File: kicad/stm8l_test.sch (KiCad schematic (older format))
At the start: 26 parts, among them J1 Conn_01x04, J2 Conn_01x02, Q1 2N7002, SW1 SW_Push, SW2 prog_sw, SW3 Rotary_Encoder_Switch, U2 STM8L101F3P, U3 BD70522GUL-E2

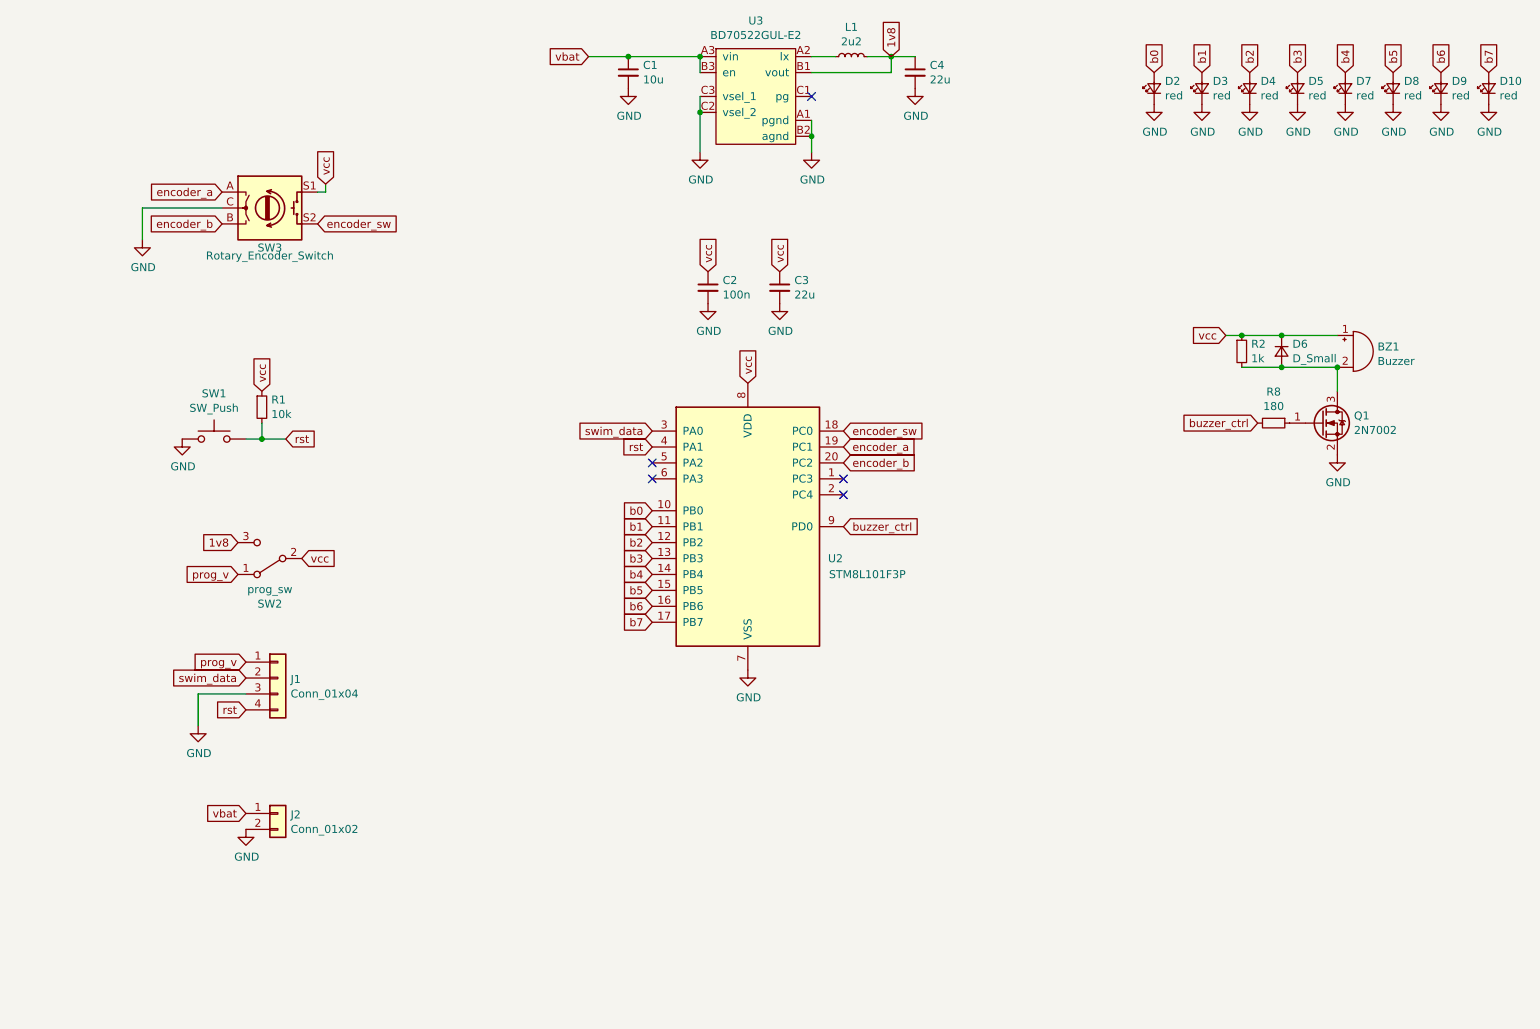
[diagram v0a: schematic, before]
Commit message: thinking about the solution, picking leds et al
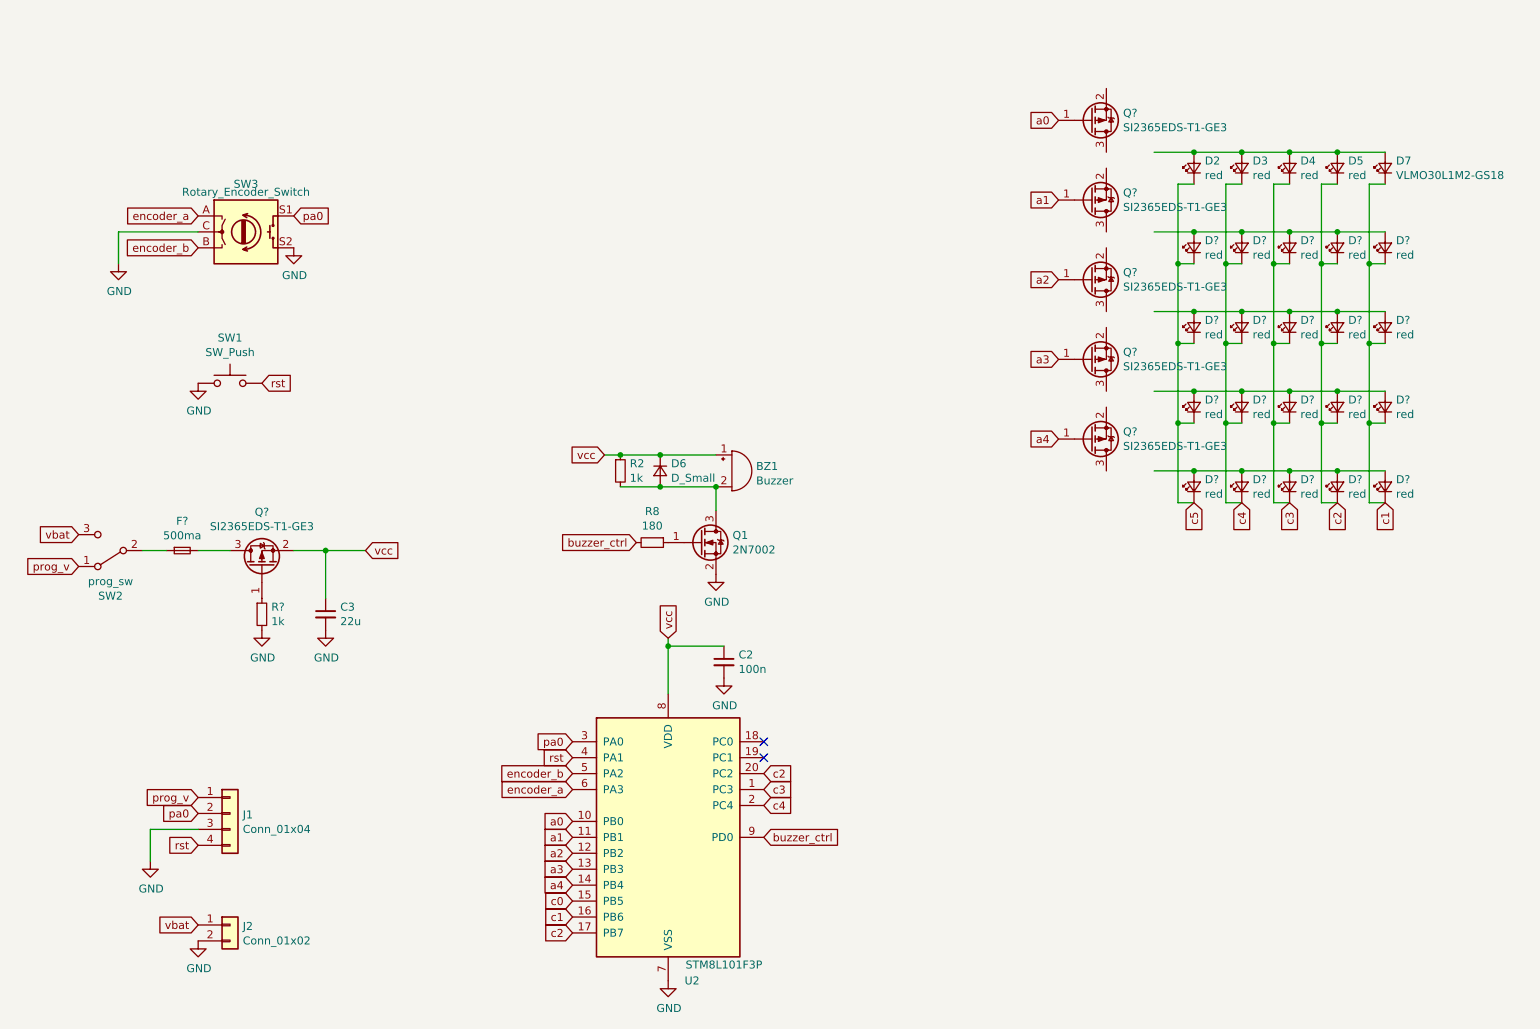
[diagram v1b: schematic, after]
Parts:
- removed C1: 10u, Capacitor_SMD:C_0805_2012Metric_Pad1.15x1.40mm_HandSolder, symbol Device:C_Small
- removed C4: 22u, Capacitor_SMD:C_0805_2012Metric_Pad1.15x1.40mm_HandSolder, symbol Device:C_Small
- removed D10, D8, D9: red, LED_SMD:LED_1206_3216Metric_Pad1.42x1.75mm_HandSolder, symbol Device:LED_Small
- removed L1: 2u2, Inductor_SMD:L_Wuerth_WE-PD-Typ-7345, symbol Device:L_Small
- removed R1: 10k, Resistor_SMD:R_0603_1608Metric_Pad1.05x0.95mm_HandSolder, symbol Device:R_Small
- removed U3: BD70522GUL-E2, good_things:BGA-9_3x3_1.76x1.56mm, symbol good_things:BD70522GUL-E2
- added D? (x20): red, LED_SMD:LED_1206_3216Metric_Pad1.42x1.75mm_HandSolder, symbol Device:LED_Small
- added F?: 500ma, symbol Device:Fuse_Small
- added Q? (x6): SI2365EDS-T1-GE3, symbol Device:Q_PMOS_GSD
- added R?: 1k, symbol Device:R_Small
- D7: value red -> VLMO30L1M2-GS18
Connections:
- net labels added: a0, a1, a2, a3, a4, c0, c1, c2, c3, c4, c5, pa0
- net labels removed: 1v8, b0, b1, b2, b3, b4, b5, b6, b7, encoder_sw, swim_data
- wire segments 27 -> 88
- no-connect marks 5 -> 2
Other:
- moved on the sheet: BZ1, C2, C3, D2, D3, D4, D5, D6, D7, J1, J2, Q1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
